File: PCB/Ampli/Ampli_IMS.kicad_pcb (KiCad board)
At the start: 2 copper layers, 67 x 32 mm, 22 parts, among them J1 5227161-3, J2 5227161-3, J3 Conn_01x03_Male, SW1 SS22D0205G2, U1 LT1464CS8, U2 LMP7721

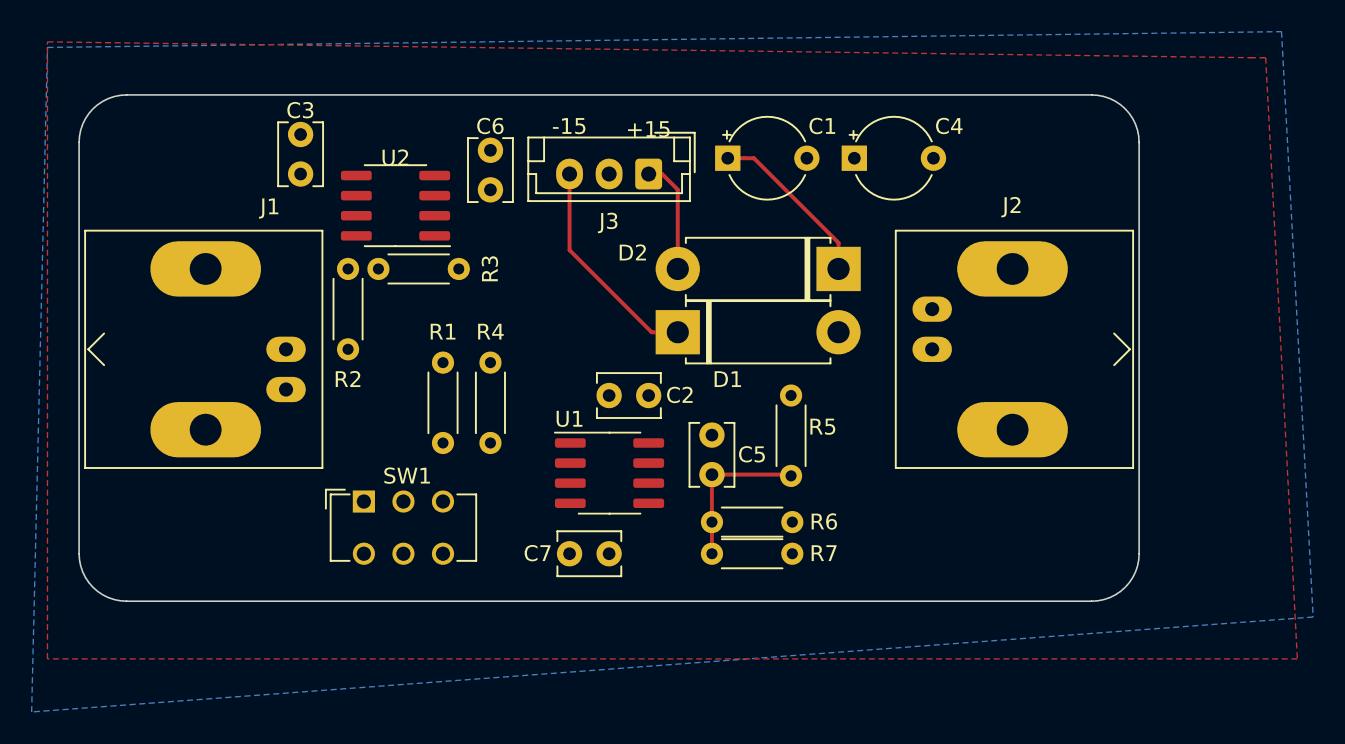
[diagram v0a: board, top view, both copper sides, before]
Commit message: tracks realised
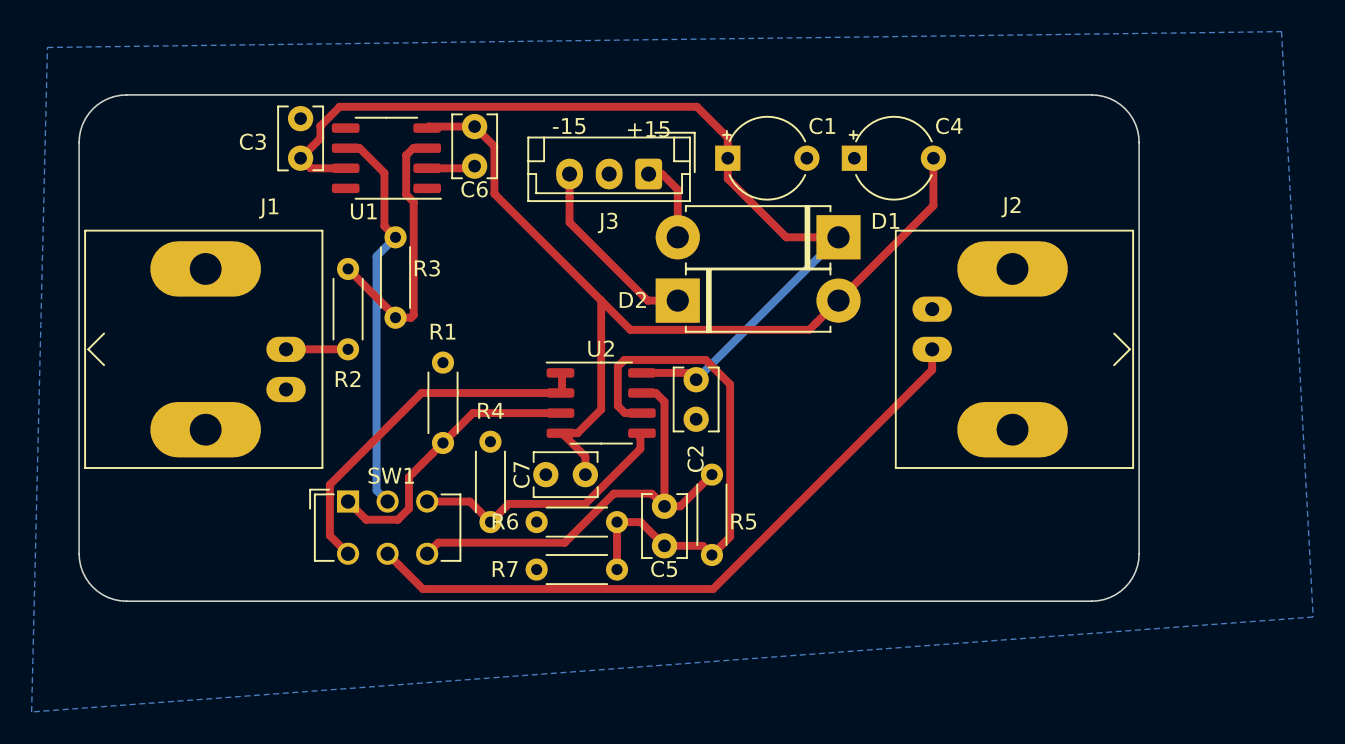
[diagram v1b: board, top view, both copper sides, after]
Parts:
- removed the U2 at (38.0, 25.0)
- added U1: ADA4625-1, Package_SO:SO-8_3.9x4.9mm_P1.27mm, F.Cu at (37.4, 22.0)
- U2: renamed from U1; footprint Package_SO:SOIC-8_3.9x4.9mm_P1.27mm -> Package_SO:SO-8_3.9x4.9mm_P1.27mm
- moved R5 7.07 mm to (58.0, 42.0)
- moved R7 6.08 mm to (52.0, 48.0), turned to 180 degrees
- moved R6 6.00 mm to (52.0, 45.0), turned to 180 degrees
- moved C5 5.41 mm to (55.0, 44.0)
- moved C7 5.10 mm to (50.0, 42.0), turned to 180 degrees
- moved R4 5.00 mm to (44.0, 45.0)
- moved R3 4.47 mm to (38.0, 27.0), turned to 270 degrees
- moved U2 4.46 mm to (51.0, 37.5)
- moved C6 4.12 mm to (43.0, 20.0), turned to 270 degrees
- moved C2 3.16 mm to (57.0, 36.0), turned to 270 degrees
- moved D1 2.00 mm to (66.0, 27.0)
- moved D2 2.00 mm to (55.8, 31.0)
- moved C3 1.00 mm to (32.0, 22.0)
- moved SW1 1.00 mm to (35.0, 43.7)
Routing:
- net /-15V: track 0.00 -> 58.6 mm
- net /+15V: track 10.9 -> 60.3 mm
- net Net-(J2-Pad1): track 0.00 -> 42.4 mm
- net Net-(C5-Pad1): track 0.00 -> 29.1 mm
- net Net-(R3-Pad1): track 0.00 -> 24.9 mm
- net Net-(SW1-Pad4): track 0.00 -> 23.2 mm
- net Net-(C5-Pad2): track 10.0 -> 33.1 mm
- net Net-(R1-Pad1): track 0.00 -> 18.0 mm
- net Net-(R2-Pad1): track 0.00 -> 17.4 mm
- net Net-(R4-Pad1): track 0.00 -> 16.9 mm
- net Net-(J1-Pad1): track 0.23 -> 4.15 mm
- net GND: track 0.00 -> 3.06 mm
- net Net-(D1-Pad2): track 7.26 -> 5.26 mm
- net Net-(D2-Pad1): track 13.8 -> 11.9 mm
- removed copper zone on F.Cu, net GND
